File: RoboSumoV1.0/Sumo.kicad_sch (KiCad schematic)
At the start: 28 parts, among them J1 BAT, J10 Conn_01x04_Pin, J2 ICSP, J4 ICSP, J5 Conn_01x06_MountingPin, J6 MotB, J7 MotA, J8 Conn_01x03_Pin, J9 I2C_Sensors, SW1 SW_SPDT, SW2 RESET, SW3 SW_DIP_x04, U1 ATmega328P-AU, U2 AMS1117-3.3, U3 TB6612FNG, Y1 20MHz

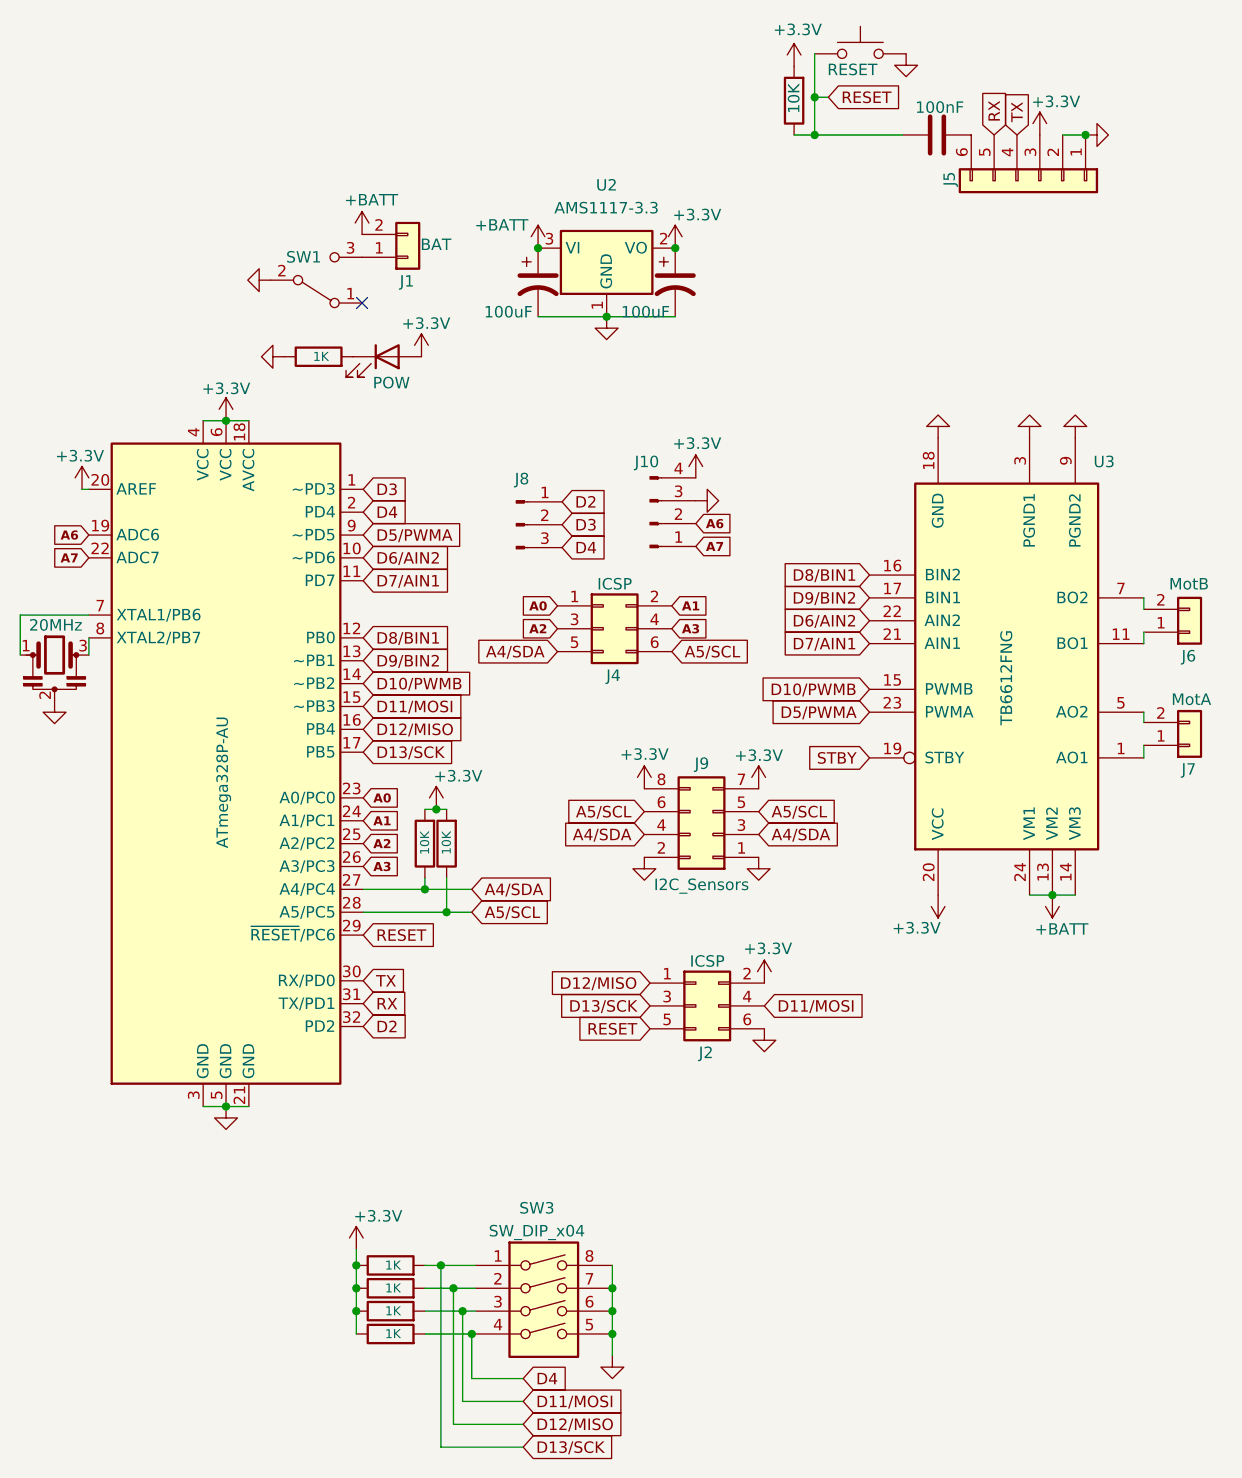
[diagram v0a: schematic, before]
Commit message: f
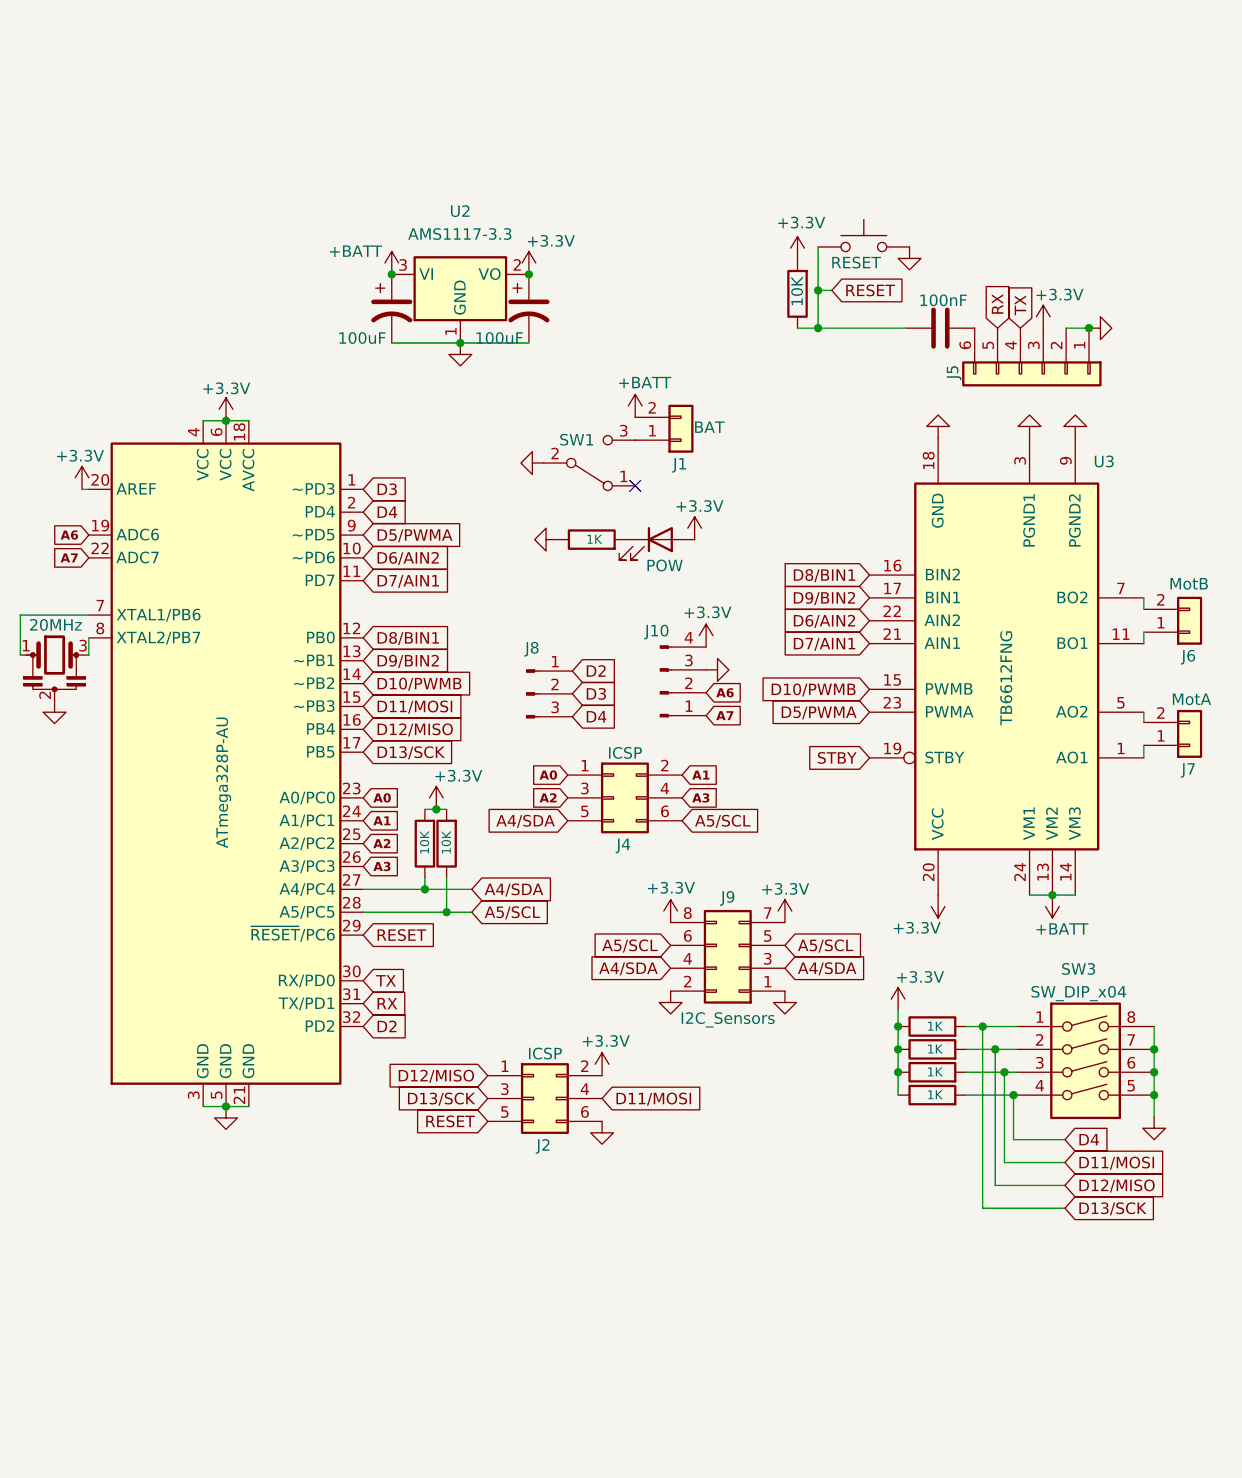
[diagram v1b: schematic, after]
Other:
- moved on the sheet: J1, J10, J2, J4, J5, J8, J9, SW1, SW3, U2
